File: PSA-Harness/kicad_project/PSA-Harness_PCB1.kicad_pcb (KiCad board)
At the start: 4 copper layers, 22.4 x 43.8 mm, 5 parts, among them J10 B2B_1, J11 B2B_2, J4 to_car_1, J5 to_car_2, J6 to_car_3

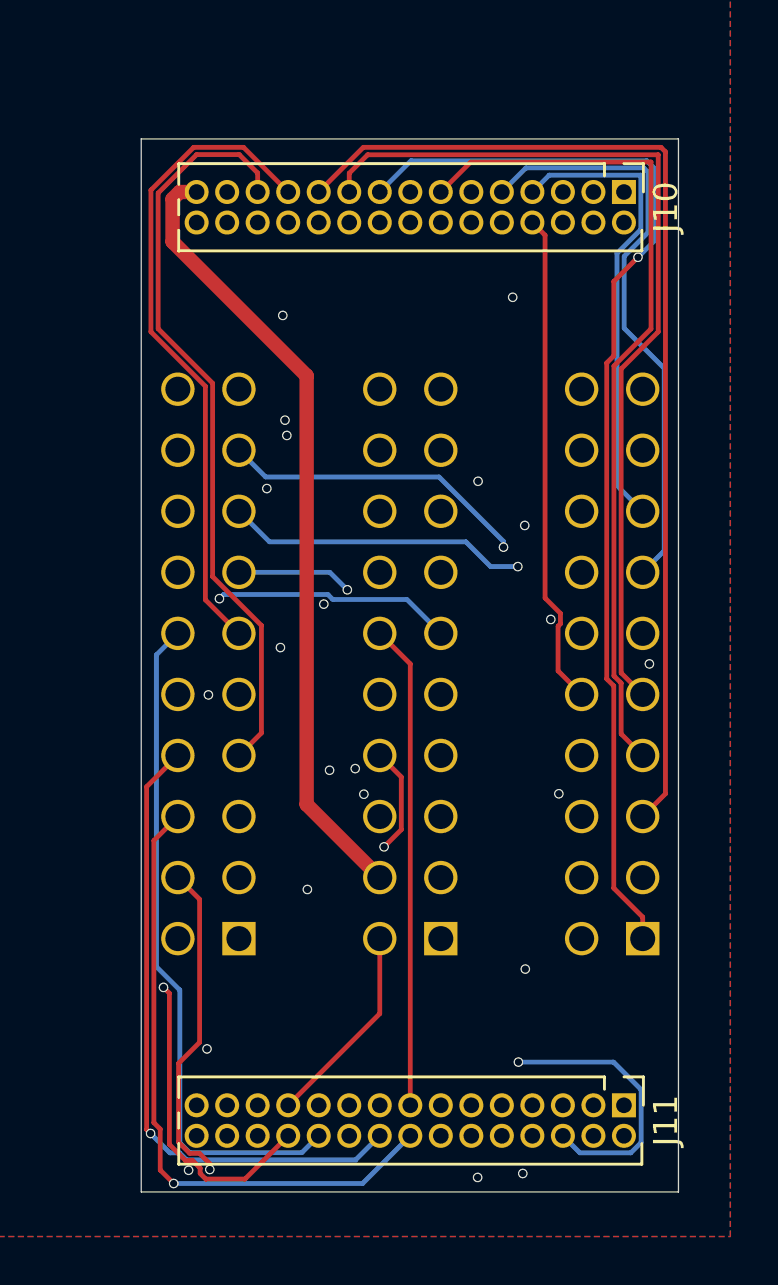
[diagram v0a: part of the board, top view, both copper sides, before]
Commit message: PCB1+2 routed
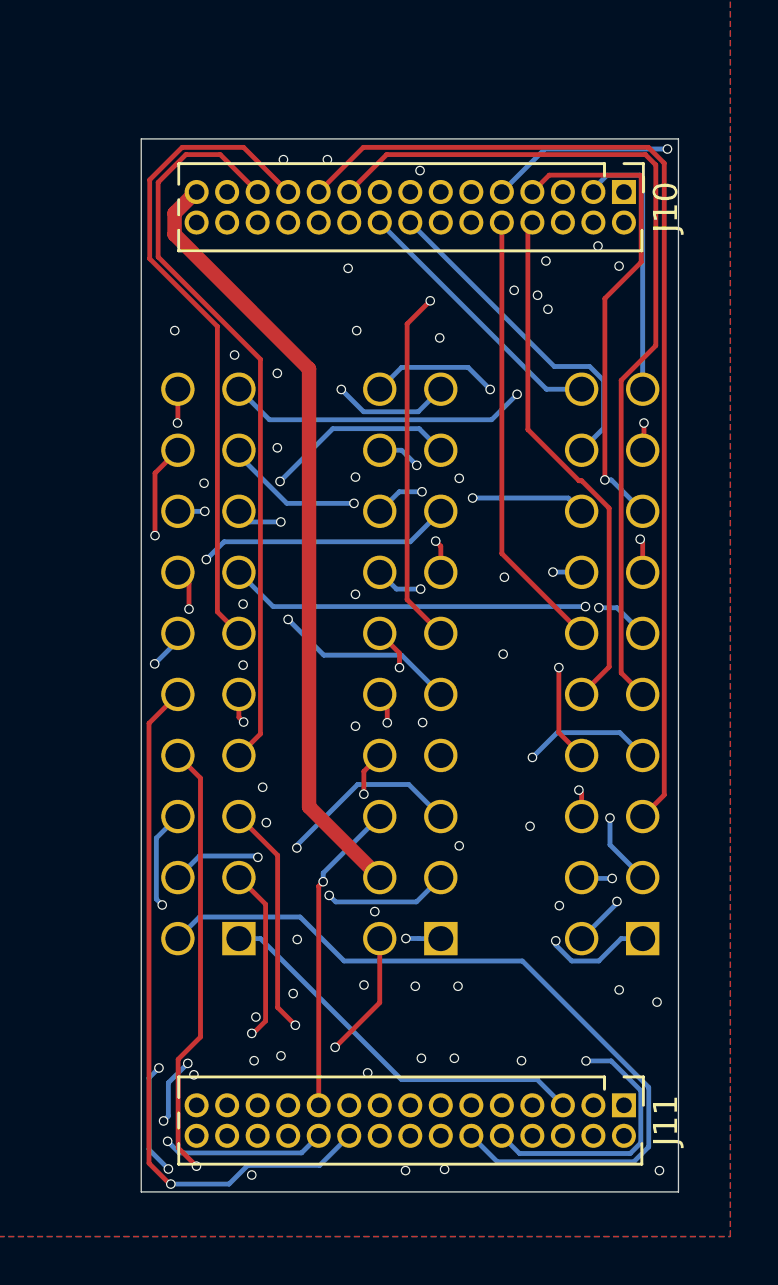
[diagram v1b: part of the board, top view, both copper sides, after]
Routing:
- net 52: track 23.9 -> 37.3 mm
- net 4: track 35.1 -> 45.2 mm, vias 0 -> 3
- net 51: track 24.1 -> 33.5 mm, vias 1 -> 0
- net 2: track 49.6 -> 41.0 mm
- net 1: track 45.6 -> 53.2 mm, vias 1 -> 2
- net 23: track 29.1 -> 33.9 mm
- net 42: track 18.7 -> 22.7 mm, vias 0 -> 1
- net 11: track 36.4 -> 32.4 mm
- net 22: track 29.9 -> 33.5 mm
- net 27: track 22.2 -> 18.8 mm, vias 0 -> 1
- net 43: track 21.5 -> 24.7 mm, vias 0 -> 1
- net 28: track 30.5 -> 33.5 mm
- net 40: track 33.0 -> 35.9 mm, vias 0 -> 1
- net 21: track 34.8 -> 32.4 mm
- net 55: track 27.2 -> 29.5 mm
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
